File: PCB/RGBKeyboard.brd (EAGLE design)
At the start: 171.4 x 114 mm, 35 parts

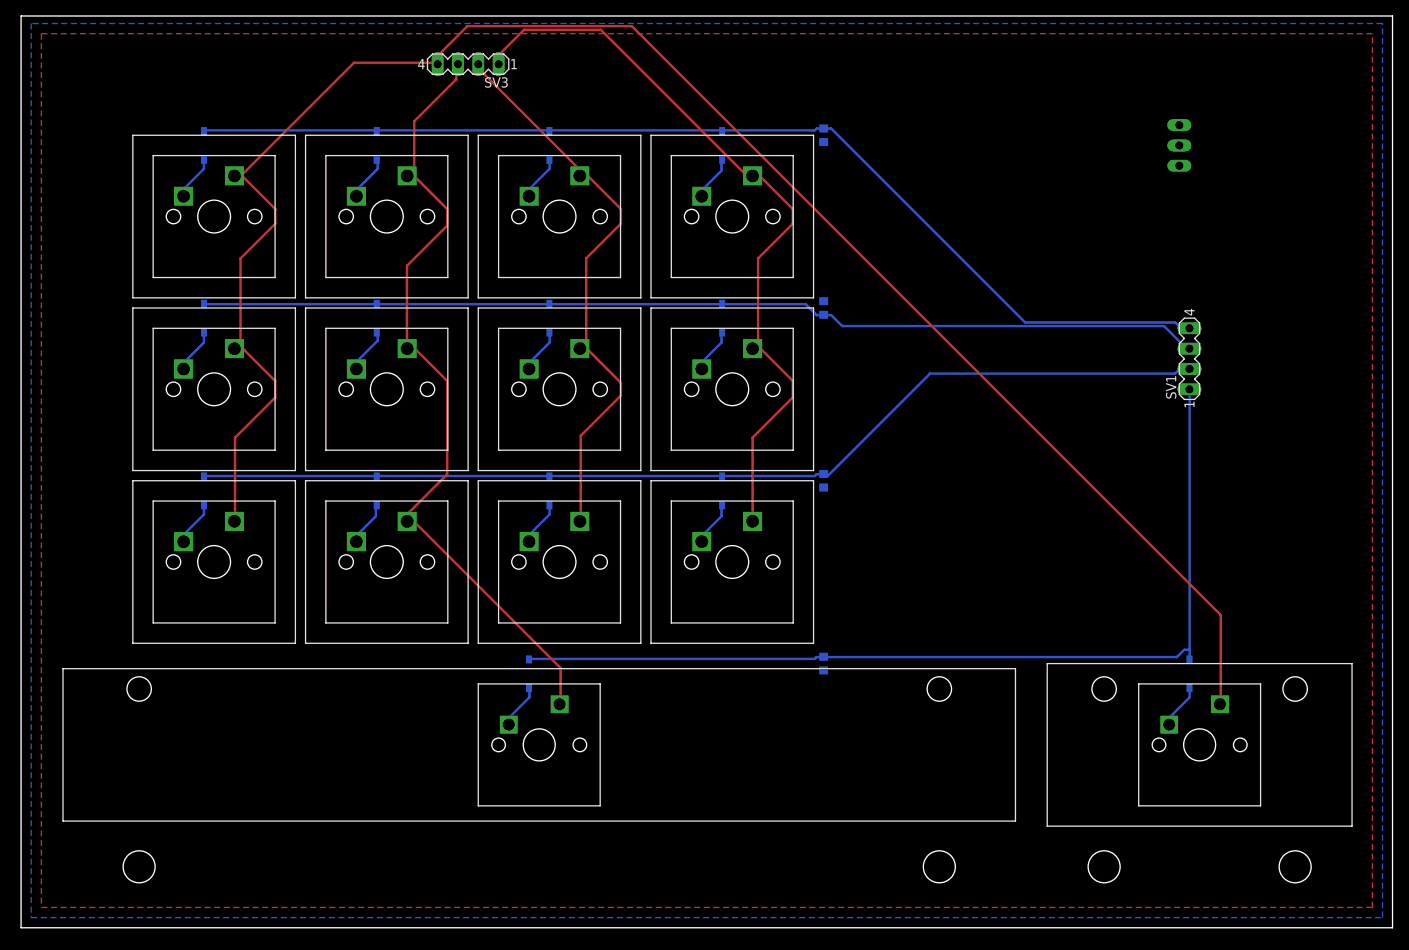
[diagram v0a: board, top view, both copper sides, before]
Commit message: New board design for 16 percent
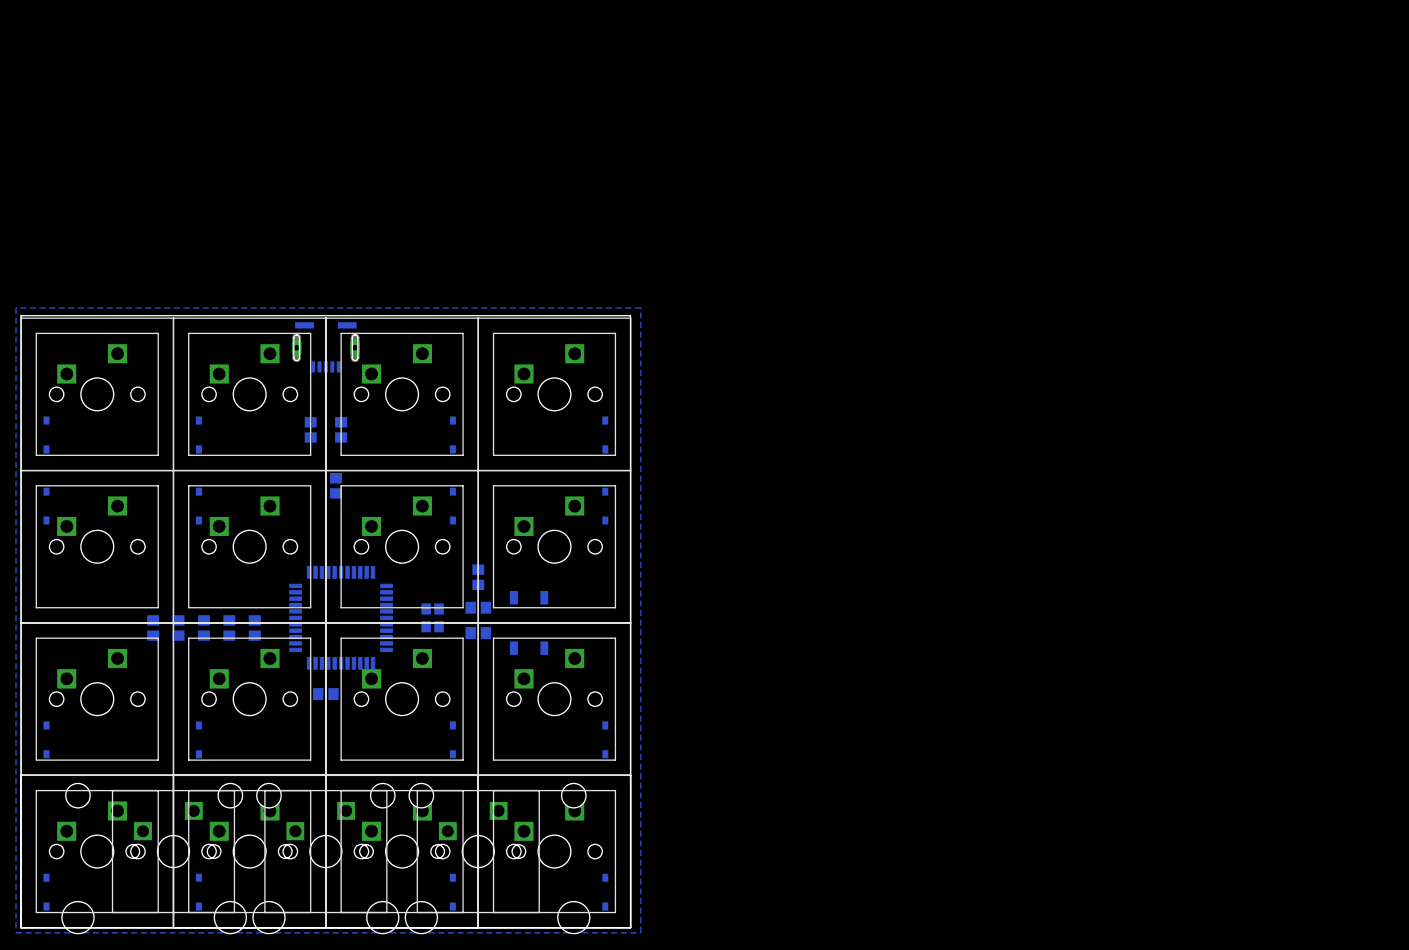
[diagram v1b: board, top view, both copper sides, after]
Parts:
- removed D14, D2: BAV21W-7-F, BAV21W-7-F:SOD3715X135N
- removed R1, R2, R3, R4: 4.7k, rcl:R0603
- removed SV1, SV3: (no value), con-lstb:MA04-1
- removed SV4: (no value), con-lstb:MA03-1
- added C1, C2, C3, C4: .1uF, rcl:C0805
- added C5, C6: 4.7uF, rcl:C0805
- added C7, C8: 22pF, rcl:C0805
- added D16, D17, D18, D19: BAV21W-7-F, BAV21W-7-F:SOD3715X135N
- added J1: UX60SC-MB-5S8, UX60SC-MB-5S8:HIROSE_UX60SC-MB-5S8
- added R5, R6: 10k, rcl:R0805
- added R7, R8: 22, rcl:R0805
- added SW1: TL3342F160QG/TR, TL3342F160QG_TR:SW_TL3342F160QG/TR
- added U$15: CHERRY_MXCHERRY_MX_1_2, CHERRY_MX:CHERRY_MX_1_2
- added U$16, U$17, U$18, U$19: CHERRY_MX, CHERRY_MX:CHERRY_MX
- added U1: ATMEGA32U4-AUR, ATMEGA32U4-AUR:QFP80P1200X1200X120-44N
- added X1: FA-238, FA-238:OSCCC320X250X70-4N
- U$14: value CHERRY_MXCHERRY_MX_1_6 -> CHERRY_MXCHERRY_MX_1_2; device CHERRY_MX:CHERRY_MX_1_6 -> CHERRY_MX:CHERRY_MX_1_2
- moved U$13 91.2 mm to (57.1, 9.53)
- moved U$14 47.6 mm to (19.1, 9.53)
- moved D3 42.5 mm to (22.2, 61.6), turned to 90 degrees
- moved D1 41.2 mm to (3.17, 61.6), turned to 90 degrees
- moved D7 39.0 mm to (73.0, 61.6), turned to 90 degrees
- moved D11 38.2 mm to (22.2, 23.5), turned to 90 degrees
- moved D6 38.2 mm to (54.0, 61.6), turned to 90 degrees
- moved D10 36.8 mm to (3.17, 23.5), turned to 90 degrees
- moved D13 34.4 mm to (73.0, 23.5), turned to 90 degrees
- moved D12 33.4 mm to (54.0, 23.5), turned to 90 degrees
- moved D5 32.3 mm to (22.2, 52.7)
- moved U$12 31.4 mm to (66.7, 66.7)
- moved D4 30.7 mm to (3.17, 52.7)
- moved U$10 29.7 mm to (66.7, 47.6)
- moved U$7 29.7 mm to (47.6, 66.7)
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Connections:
- removed net COL2: SV3.2, U$7.2, U$8.2, U$9.2
- removed net DVCC: SV4.3
- removed net N$4: D2.A, U$13.1
- removed net N$5: D14.A, U$14.1
- new net N$10: R6.2, U1.33
- new net N$13: J1.1, U1.2
- new net N$14: R7.2, U1.3
- new net N$15: J1.2, R7.1
- new net N$16: R8.2, U1.4
- new net N$17: J1.3, R8.1
- new net N$18: D17.A, U$14.1, U$18.1
- new net N$19: D19.A, U$16.1
- new net N$20: D16.A, U$13.1, U$17.1
- new net N$21: D18.A, U$15.1, U$19.1
- new net N$22: U$10.2, U$11.2, U$12.2, U$16.2
- new net N$7: C8.2, U1.17, X1.3
- new net N$8: C7.2, U1.16, X1.1
- new net N$9: R5.1, SW1.1, SW1.2, U1.13
- new net UCAP: C6.2, U1.6
- new net VCC: C1.1, C2.1, C3.1, C4.1, C5.1, R5.2, U1.14, U1.24, U1.34, U1.44, U1.7
- net COL0: now also U$17.2; no longer SV3.4
- net COL1: now also U$18.2; no longer SV3.3
- net COL3: now also U$15.2, U$19.2, U$7.2, U$8.2, U$9.2; no longer SV3.1, U$10.2, U$11.2, U$12.2
- net GND: now also C1.2, C2.2, C3.2, C4.2, C5.2, C6.1, C7.1, C8.1, J1.5, J1.S1, J1.S2, J1.S3, J1.S4, R6.1, SW1.3, SW1.4, U1.15, U1.23, U1.35, U1.43, U1.5, X1.2, X1.4; no longer R1.1, R2.1, R3.1, R4.1, SV4.2
- net ROW0: no longer R1.2, SV1.4
- net ROW1: no longer R2.2, SV1.3
- net ROW2: no longer R3.2, SV1.2
- net ROW3: now also D16.C, D17.C, D18.C, D19.C; no longer D14.C, D2.C, R4.2, SV1.1
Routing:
- net COL0: track 227.1 -> 0.00 mm
- net ROW0: track 133.9 -> 0.00 mm
- net ROW2: track 129.1 -> 0.00 mm
- net ROW1: track 125.6 -> 0.00 mm
- net ROW3: track 116.9 -> 0.00 mm
- net COL1: track 100.6 -> 0.00 mm
- net COL3: track 95.2 -> 0.00 mm
- net COL2: track 72.6 -> 0.00 mm
- net N$6: track 5.78 -> 0.00 mm
- net N$2: track 5.73 -> 0.00 mm
- net N$3: track 5.69 -> 0.00 mm
- net N$5: track 5.65 -> 0.00 mm
- net N$11: track 5.65 -> 0.00 mm
- net N$33: track 5.64 -> 0.00 mm
- net N$12: track 5.64 -> 0.00 mm
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- removed copper zone on layer 1, net GND
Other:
- board size 171.4 x 114 mm -> 76.2 x 76.5 mm
